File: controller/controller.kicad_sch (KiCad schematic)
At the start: 74 parts, among them SW1 SW_SPDT, SW2 SW_SPST

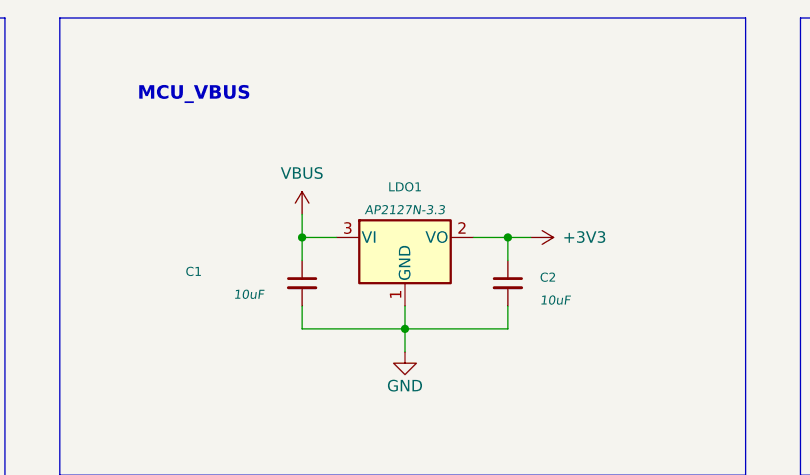
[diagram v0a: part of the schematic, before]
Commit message: Sensor v1
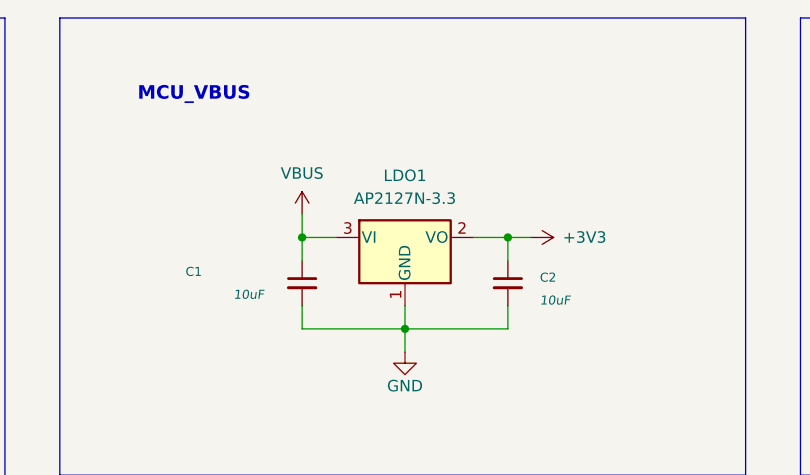
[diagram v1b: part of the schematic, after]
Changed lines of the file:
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@@
     (pin "9")
+  )
+  (symbol (lib_id "Regulator_Linear:AP2127N-3.3") (at 138.684 42.418 0) (unit 1)
+    (in_bom yes) (on_board yes) (fields_autoplaced)
+    (property "Reference" "LDO1" (id 0) (at 138.684 35.56 0))
+    (property "Value" "AP2127N-3.3" (id 1) (at 138.684 38.1 0))
+    (property "Footprint" "Package_TO_SOT_SMD:SOT-23" (id 2) (at 138.684 36.703 0)
+      (effects (font (size 1.27 1.27) italic) hide)
+    )
+    (property "Datasheet" "https://www.diodes.com/assets/Datasheets/AP2127.pdf" (id 3) (at 138.684 42.418 0)
+      (effects (font (size 1.27 1.27)) hide)
+    )
+    (pin "1")
+    (pin "2")
+    (pin "3")
   )
   (symbol (lib_id "Device:C_Small") (at 440.182 50.419 0) (unit 1)
@@
     (pin "6")
   )
-  (symbol (lib_id "Regulator_Linear:AP2127N-3.3") (at 138.684 42.418 0) (unit 1)
-    (in_bom yes) (on_board yes) (fields_autoplaced)
-    (property "Reference" "LDO1" (id 0) (at 138.684 36.83 0)
-      (effects (font (size 1 1)))
-    )
-    (property "Value" "AP2127N-3.3" (id 1) (at 138.684 39.37 0)
-      (effects (font (size 1 1) italic))
-    )
-    (property "Footprint" "Package_TO_SOT_SMD:SOT-23" (id 2) (at 138.684 36.703 0)
-      (effects (font (size 1.27 1.27) italic) hide)
-    )
-    (property "Datasheet" "https://www.diodes.com/assets/Datasheets/AP2127.pdf" (id 3) (at 138.684 42.418 0)
-      (effects (font (size 1.27 1.27)) hide)
-    )
-    (pin "1")
-    (pin "2")
-    (pin "3")
-  )
   (symbol (lib_id "Connector_Generic:Conn_01x05") (at 340.36 373.634 0) (unit 1)
     (in_bom yes) (on_board yes) (fields_autoplaced)
@@
       (reference "H14") (unit 1) (value "Conn_01x03") (footprint "Connector_Molex:Molex_PicoBlade_53047-0310_1x03_P1.25mm_Vertical")
     )
-    (path "/c43cde42-06c8-4a38-a840-be919d24617a"
+    (path "/082fbcf6-a43d-4e76-ba92-bf94710b0792"
       (reference "LDO1") (unit 1) (value "AP2127N-3.3") (footprint "Package_TO_SOT_SMD:SOT-23")
     )

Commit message: start work on host mcu
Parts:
- FB1: footprint Inductor_SMD:L_1206_3216Metric -> Inductor_SMD:L_0603_1608Metric
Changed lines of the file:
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@@
     (property "Reference" "FB1" (id 0) (at 316.0649 35.56 90))
     (property "Value" "120R" (id 1) (at 316.0649 38.1 90))
-    (property "Footprint" "Inductor_SMD:L_1206_3216Metric" (id 2) (at 316.103 43.942 90)
+    (property "Footprint" "Inductor_SMD:L_0603_1608Metric" (id 2) (at 316.103 43.942 90)
       (effects (font (size 1.27 1.27)) hide)
     )
@@
     )
     (path "/8b4289f2-9a86-4728-acfc-6857feae1132"
-      (reference "FB1") (unit 1) (value "120R") (footprint "Inductor_SMD:L_1206_3216Metric")
+      (reference "FB1") (unit 1) (value "120R") (footprint "Inductor_SMD:L_0603_1608Metric")
     )
     (path "/c36b3a61-3f93-4a26-bac4-d190cb007fea"
